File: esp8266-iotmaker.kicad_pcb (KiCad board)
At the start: 2 copper layers, 49 parts, among them J1 CONN_01X10, J2 CONN_01X10, Q1 S8050, Q2 S8050, SW1 SW_Push, SW2 SW_Push, U1 usb_mini_b, U2 chip-esp8266, U3 CP2102, U4 25Q32, U6 AMS1117-3.3, Y1 26MHz

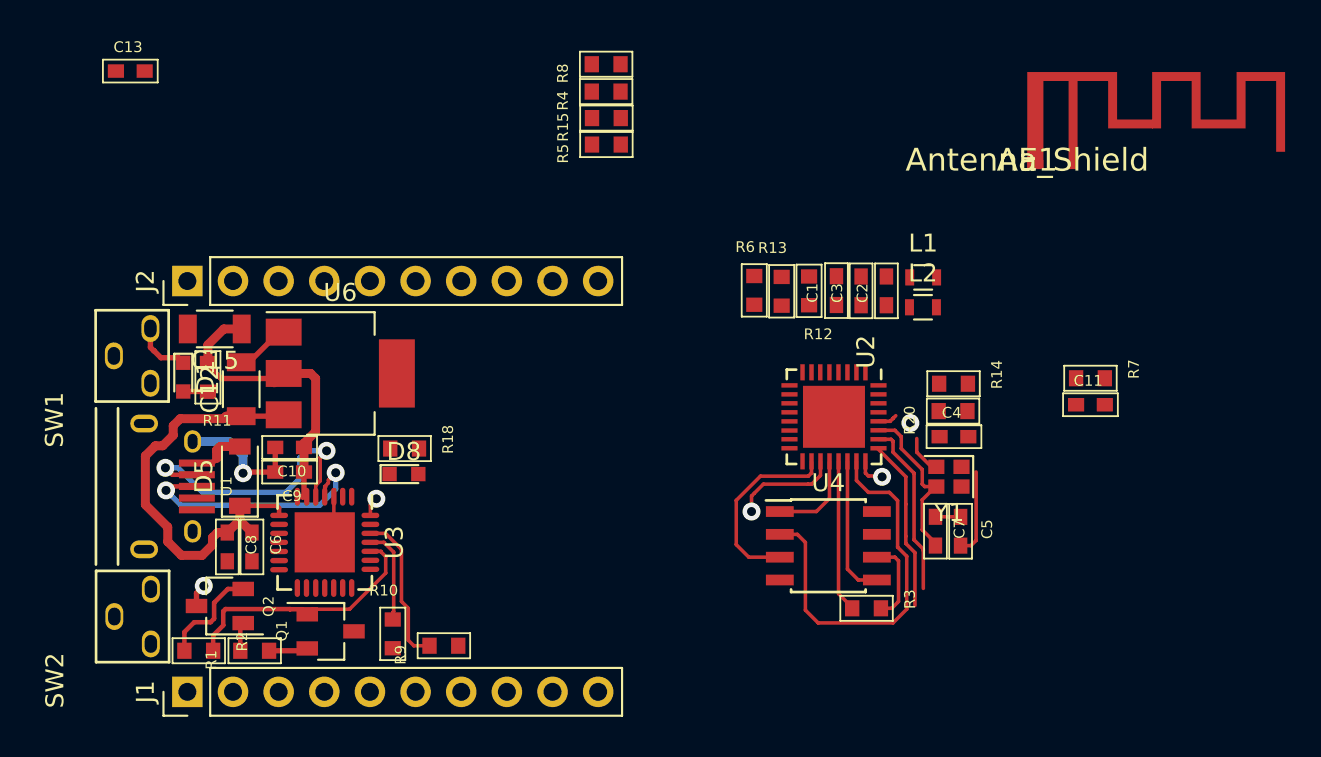
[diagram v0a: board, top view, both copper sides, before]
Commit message: complete pcb ver2.0
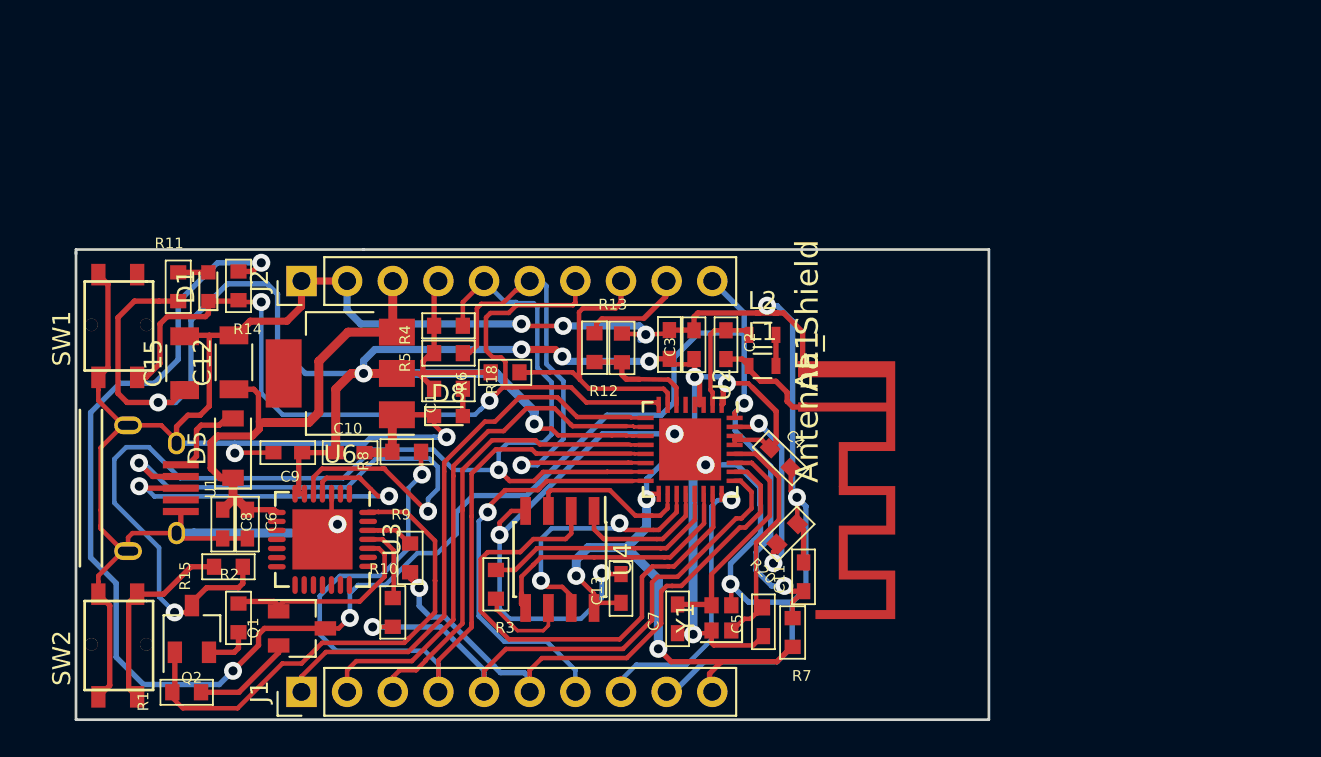
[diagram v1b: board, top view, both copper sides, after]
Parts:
- SW1, SW2: footprint esp8266:tactile switches -> esp8266:nut_nhan_ngang
- moved R14 40.2 mm to (98.1, 74.8), turned to 270 degrees
- moved C13 39.7 mm to (119.4, 91.6), turned to 90 degrees
- moved R15 32.6 mm to (97.5, 90.4)
- moved R8 24.3 mm to (107.5, 84.0)
- moved R7 21.8 mm to (128.9, 94.1), turned to 270 degrees
- moved R3 20.7 mm to (112.4, 91.4), turned to 270 degrees
- moved C11 18.6 mm to (129.5, 91.0), turned to 90 degrees
- moved AE1 16.6 mm to (129.7, 79.0), turned to 270 degrees
- moved R4 15.7 mm to (109.8, 77.0)
- moved C7 15.2 mm to (122.5, 93.3), turned to 90 degrees
- moved U4 15.0 mm to (116.0, 90.0), turned to 270 degrees
- moved Y1 14.9 mm to (125.0, 93.3), turned to 90 degrees
- moved R6 14.6 mm to (112.9, 79.6), turned to 180 degrees
- moved R5 14.6 mm to (109.8, 78.5)
- moved R12 12.3 mm to (117.9, 78.2)
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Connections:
- J2 pad 1: GPIO16 -> GND
- J2 pad 10: GND -> REST
- J2 pad 2: ADC_EX -> GND
- J2 pad 3: GND -> VCC
- J2 pad 5: EN -> GPIO0
- J2 pad 6: REST -> GPIO2
- J2 pad 7: GPIO0 -> GPIO16
- J2 pad 8: GPIO2 -> EN
- J2 pad 9: VUSB -> ADC_EX
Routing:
- net GND: track 16.3 -> 236.2 mm, vias 1 -> 14
- net 3V3: track 18.2 -> 146.5 mm, vias 0 -> 11
- net REST: track 0.00 -> 101.6 mm, vias 0 -> 5
- net GPIO0: track 1.29 -> 66.8 mm, vias 1 -> 2
- net GPIO16: track 3.23 -> 50.5 mm, vias 0 -> 2
- net GPIO15: track 0.00 -> 46.1 mm, vias 0 -> 1
- net GPIO14: track 0.00 -> 32.4 mm
- net GPIO12: track 0.00 -> 29.3 mm
- net GPIO2: track 0.00 -> 27.8 mm, vias 0 -> 1
- net DTR: track 2.67 -> 28.4 mm, vias 1 -> 0
- net GPIO13: track 0.00 -> 25.5 mm
- net TXD: track 9.74 -> 33.6 mm, vias 0 -> 1
- net GPIO4: track 0.00 -> 23.5 mm, vias 0 -> 1
- net RXD: track 9.68 -> 32.7 mm, vias 0 -> 1
- net EN: track 0.00 -> 17.2 mm
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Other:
- board outline added: 50.8 x 26.2 mm
- net class Default: clearance 0.2 -> 0.254
- rule trace_clearance: 0.2 -> 0.254
